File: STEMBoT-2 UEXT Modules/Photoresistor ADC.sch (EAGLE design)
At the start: 19 parts, among them IC1 74HC165PW,118, IC2 LMV324DR2G, IC3 LMV324DR2G, Q1 MMBT3904LP-7, U1 SN74HC148D

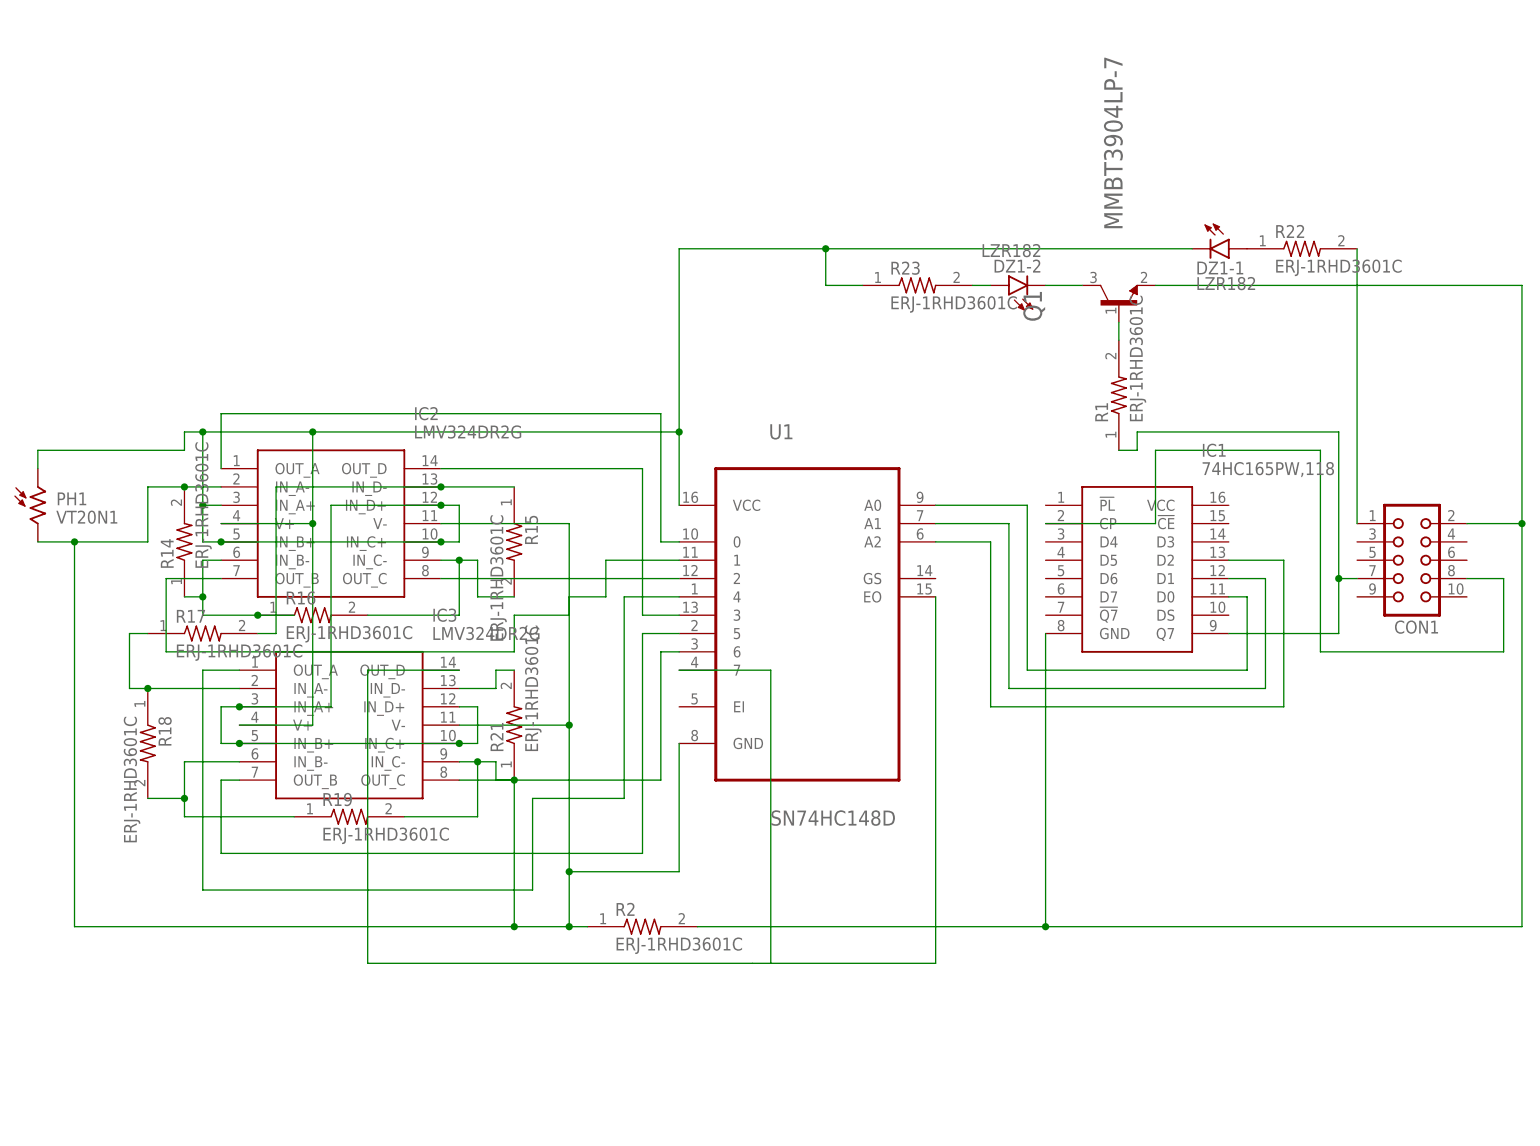
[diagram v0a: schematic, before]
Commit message: Once again, updating ADC shematics and boards. Used autorouter.
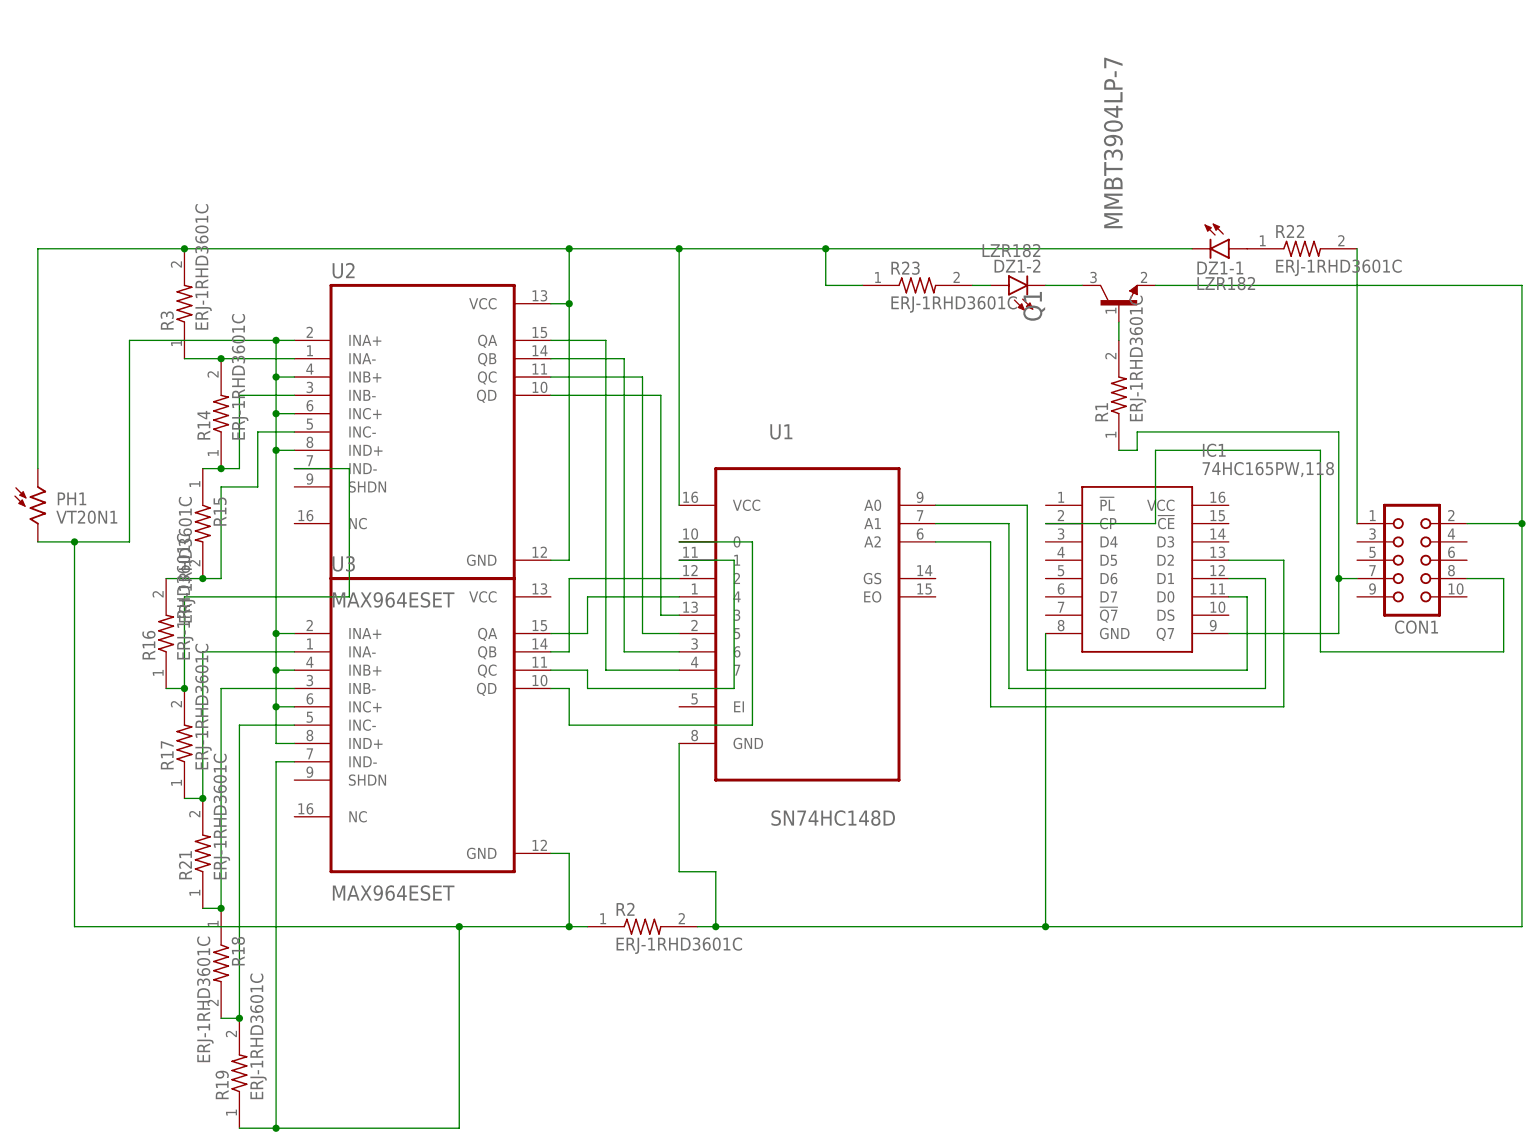
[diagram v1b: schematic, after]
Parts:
- removed IC2, IC3: LMV324DR2G, LMV324DR2G:LMV324DR2G
- added R3: ERJ-1RHD3601C, Resistor:ERJ-1RHD3601C
- added U2, U3: MAX964ESET, MAX964ESET:MAX964ESET
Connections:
- removed net N$2: IC2.OUT_B, U1.1
- removed net N$30: IC2.OUT_D, U1.3
- removed net N$31: IC2.OUT_C, U1.2
- removed net N$33: IC2.OUT_A, U1.0
- new net N$17: U1.6, U2.QB
- new net N$18: U1.5, U2.QC
- new net N$27: U1.2, U3.QB
- new net N$28: U1.1, U3.QC
- new net N$29: U1.0, U3.QD
- net N$10: now also R17.2, U2.IND-; no longer IC2.IN_B-, R14.1
- net N$11: now also R17.1, R21.2, U3.INA-; no longer IC3.OUT_C, U1.6
- net N$12: now also R3.2, U2.GND, U2.VCC; no longer IC2.IN_A+, IC2.IN_B+, IC2.IN_C+, IC2.IN_D+, IC2.V+, IC3.IN_A+, IC3.IN_B+, IC3.IN_C+, IC3.IN_D+, IC3.V+
- net N$13: now also R18.1, R21.1, U3.INB-; no longer IC2.IN_C-, R15.2, R16.2
- net N$14: now also R18.2, R19.2, U3.INC-; no longer IC2.IN_D-, R15.1, R17.2
- net N$15: now also PH1.2, R19.1, R2.1, U2.INA+, U2.INB+, U2.INC+, U2.IND+, U3.GND, U3.INA+, U3.INB+, U3.INC+, U3.IND+, U3.IND-; no longer IC3.IN_D-, R21.2
- net N$16: now also U2.QA; no longer IC3.OUT_D, U1.EO
- net N$22: now also U1.GND
- net N$23: now also U1.3, U2.QD; no longer IC3.OUT_B, U1.5
- net N$26: now also U3.QA; no longer IC3.OUT_A
- net N$3: now also R15.2, R16.2, U2.INC-; no longer IC3.IN_A-, R17.1, R18.1
- net N$8: now also R3.1, U2.INA-; no longer IC2.IN_A-, IC2.V-, IC3.IN_C-, IC3.V-, PH1.2, R19.2, R2.1, R21.1, U1.GND
- net N$9: now also R14.1, R15.1, U2.INB-; no longer IC3.IN_B-, R18.2, R19.1
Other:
- moved on the sheet: R14, R15, R16, R17, R18, R19, R21
